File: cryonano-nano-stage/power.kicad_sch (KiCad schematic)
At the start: 35 parts, among them Q1 PMV100EPAR, U4 AP7363-33D-13

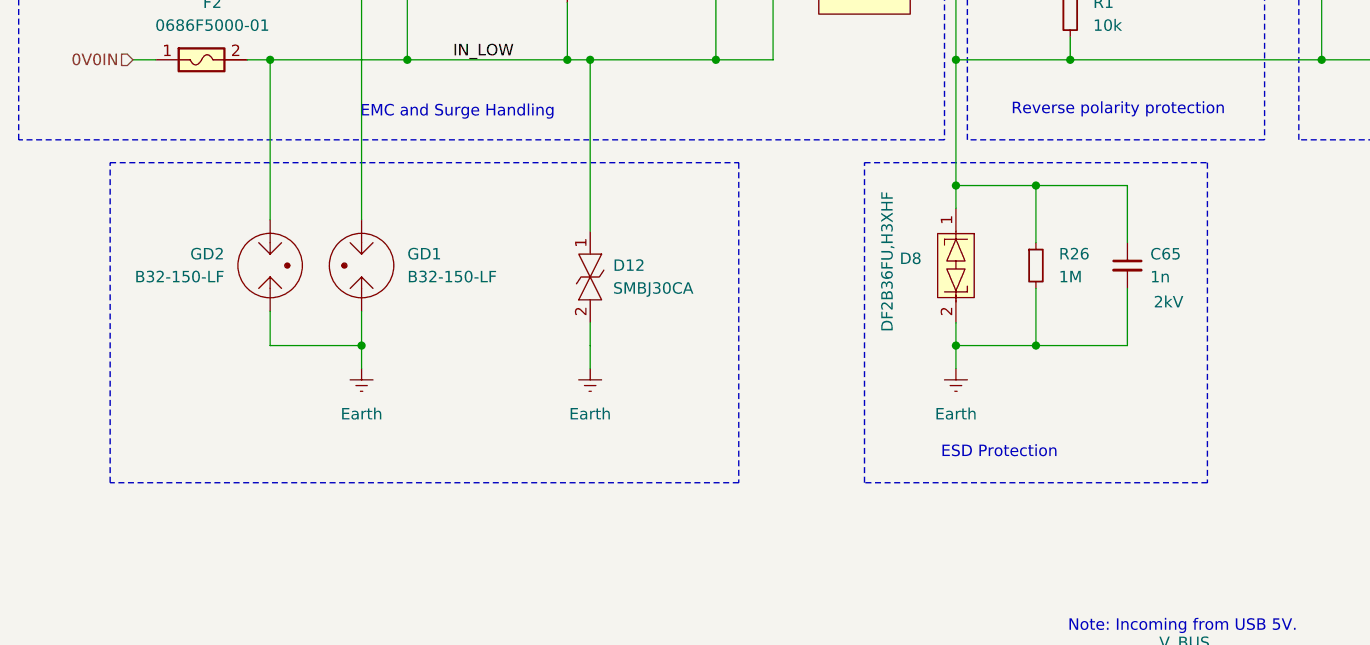
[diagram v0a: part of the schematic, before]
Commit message: drc ok, review schematic
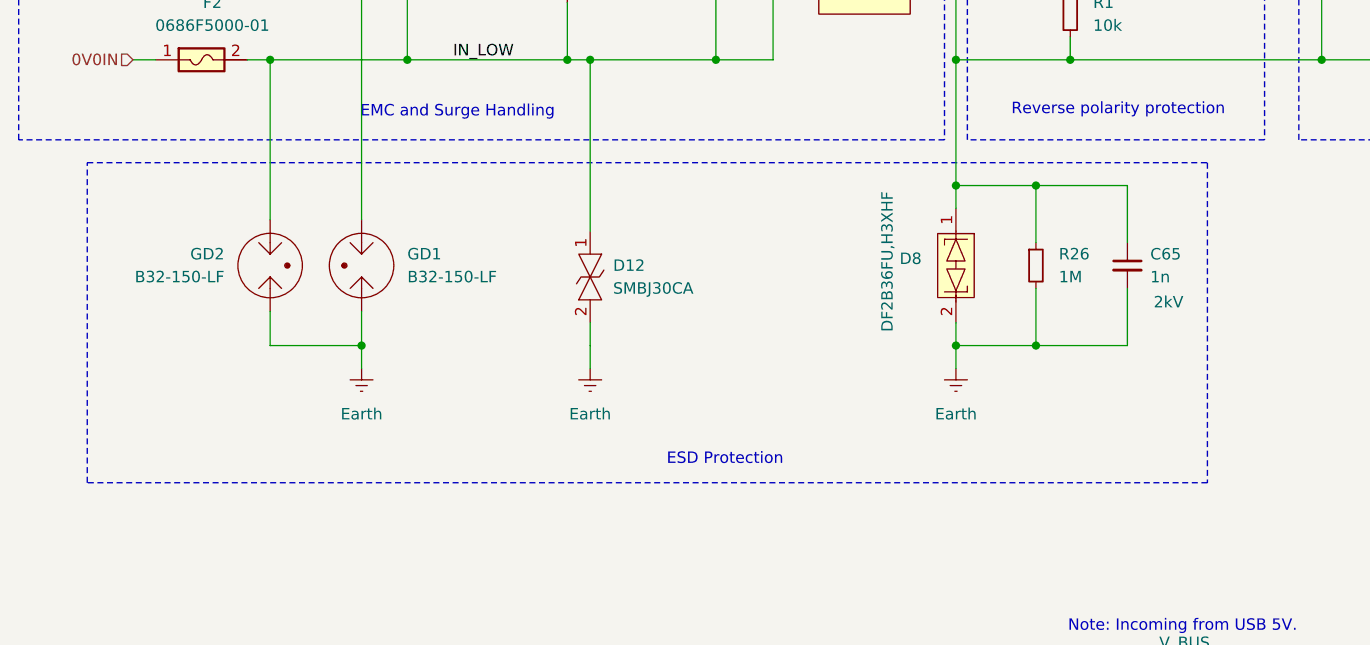
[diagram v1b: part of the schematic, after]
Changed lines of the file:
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@@
-	)
-	(rectangle
-		(start 35.56 68.58)
-		(end 105.41 104.14)
-		(stroke
-			(width 0.1524)
-			(type dash)
-		)
-		(fill
-			(type none)
-		)
 	)
 	(rectangle
@@
 	)
 	(rectangle
-		(start 119.38 68.58)
+		(start 33.02 68.58)
 		(end 157.48 104.14)
 		(stroke
@@
 	(text "ESD Protection"
 		(exclude_from_sim no)
-		(at 134.366 100.838 0)
+		(at 103.886 101.6 0)
 		(effects
 			(font
